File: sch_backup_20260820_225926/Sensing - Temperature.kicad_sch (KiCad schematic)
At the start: 8 parts, among them U16 SHT40-N-NF, U17 SHT40-N-NF

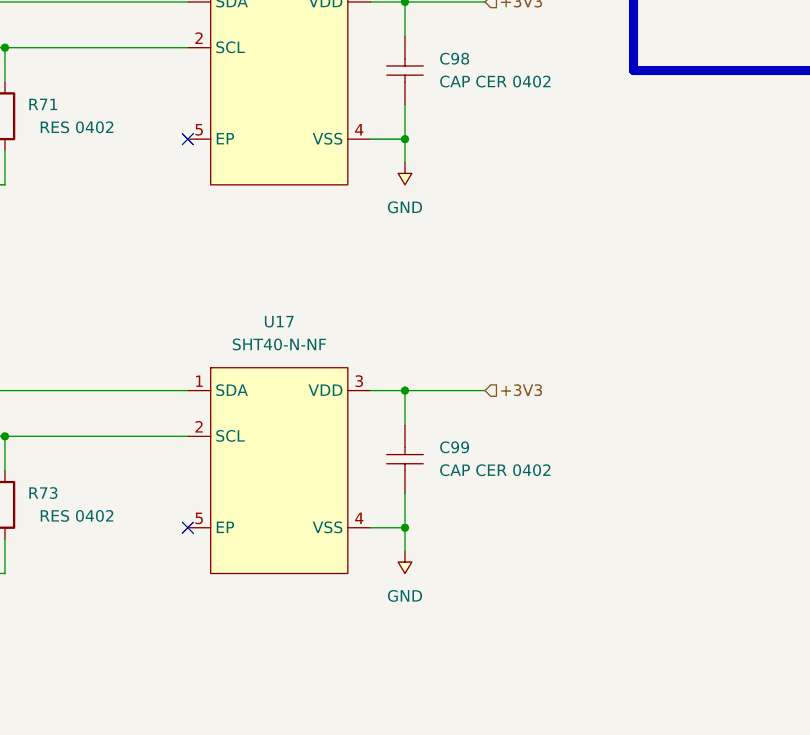
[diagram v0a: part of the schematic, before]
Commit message: Update Schematic
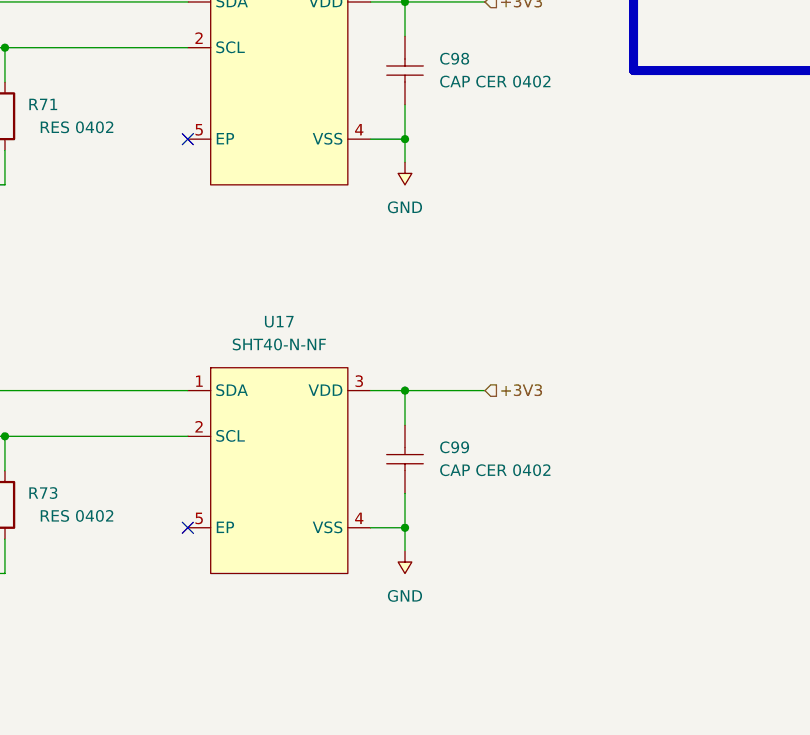
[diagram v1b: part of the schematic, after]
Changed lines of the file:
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@@
 	(symbol
 		(lib_id "Power_symbols:GND")
-		(at 167.64 80.01 0)
+		(at 165.1 78.74 180)
 		(unit 1)
 		(exclude_from_sim no)
@@
 		(dnp no)
 		(fields_autoplaced yes)
-		(property "Reference" "#PWR0133"
-			(at 167.386 71.374 0)
+		(property "Reference" "#PWR129"
+			(at 165.1 78.74 0)
 			(do_not_autoplace yes)
 			(effects
@@
 		)
 		(property "Footprint" ""
-			(at 167.64 80.01 0)
+			(at 165.1 78.74 0)
 			(effects
 				(font
@@
 		)
 		(property "Datasheet" ""
-			(at 167.64 80.01 0)
+			(at 165.1 78.74 0)
 			(effects
 				(font
@@
 		)
 		(property "Description" "Power Symbol - Global Ground"
-			(at 167.64 86.868 0)
-			(effects
-				(font
-					(size 1.27 1.27)
-				)
-				(hide yes)
-			)
-		)
-		(pin "1"
-		)
-		(instances
-			(project "Master_Hand_Kicad"
-				(path "/f9e05184-c88b-4a88-ae9c-ab2bdb32be7c/c5103ceb-5325-4a84-a025-9638a412984e/2e63ad8d-085e-4704-a18e-2216b579ffe6"
-					(reference "#PWR0133")
+			(at 165.1 78.74 0)
+			(effects
+				(font
+					(size 1.27 1.27)
+				)
+				(hide yes)
+			)
+		)
+		(pin "1"
+		)
+		(instances
+			(project "Master_Hand_Kicad"
+				(path "/f9e05184-c88b-4a88-ae9c-ab2bdb32be7c/c5103ceb-5325-4a84-a025-9638a412984e/2e63ad8d-085e-4704-a18e-2216b579ffe6"
+					(reference "#PWR129")
 					(unit 1)
 				)
@@
 	(symbol
 		(lib_id "Power_symbols:GND")
-		(at 167.64 123.19 0)
+		(at 165.1 121.92 180)
 		(unit 1)
 		(exclude_from_sim no)
@@
 		(dnp no)
 		(fields_autoplaced yes)
-		(property "Reference" "#PWR0134"
-			(at 167.386 114.554 0)
+		(property "Reference" "#PWR130"
+			(at 165.1 121.92 0)
 			(do_not_autoplace yes)
 			(effects
@@
 		)
 		(property "Footprint" ""
-			(at 167.64 123.19 0)
+			(at 165.1 121.92 0)
 			(effects
 				(font
@@
 		)
 		(property "Datasheet" ""
-			(at 167.64 123.19 0)
+			(at 165.1 121.92 0)
 			(effects
 				(font
@@
 		)
 		(property "Description" "Power Symbol - Global Ground"
-			(at 167.64 130.048 0)
-			(effects
-				(font
-					(size 1.27 1.27)
-				)
-				(hide yes)
-			)
-		)
-		(pin "1"
-		)
-		(instances
-			(project "Master_Hand_Kicad"
-				(path "/f9e05184-c88b-4a88-ae9c-ab2bdb32be7c/c5103ceb-5325-4a84-a025-9638a412984e/2e63ad8d-085e-4704-a18e-2216b579ffe6"
-					(reference "#PWR0134")
-					(unit 1)
-				)
+			(at 165.1 121.92 0)
+			(effects
+				(font
+					(size 1.27 1.27)
+				)
+				(hide yes)
+			)
+		)
+		(pin "1"
+		)
+		(instances
+			(project "Master_Hand_Kicad"
+				(path "/f9e05184-c88b-4a88-ae9c-ab2bdb32be7c/c5103ceb-5325-4a84-a025-9638a412984e/2e63ad8d-085e-4704-a18e-2216b579ffe6"
+					(reference "#PWR130")
+					(unit 1)
+				)
